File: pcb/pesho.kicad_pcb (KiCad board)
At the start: 2 copper layers, 132.5 x 65 mm, 60 parts, among them IC1 4N25, IC2 4N25, IC3 4N25, IC4 4N25, IC5 4N25, IC6 4N25, P1 Power, P2 Bulkey, P3 Raspberry Pi CONN, P4 Serial, U1 JE-112D, U2 JE-112D, U3 JE-112D

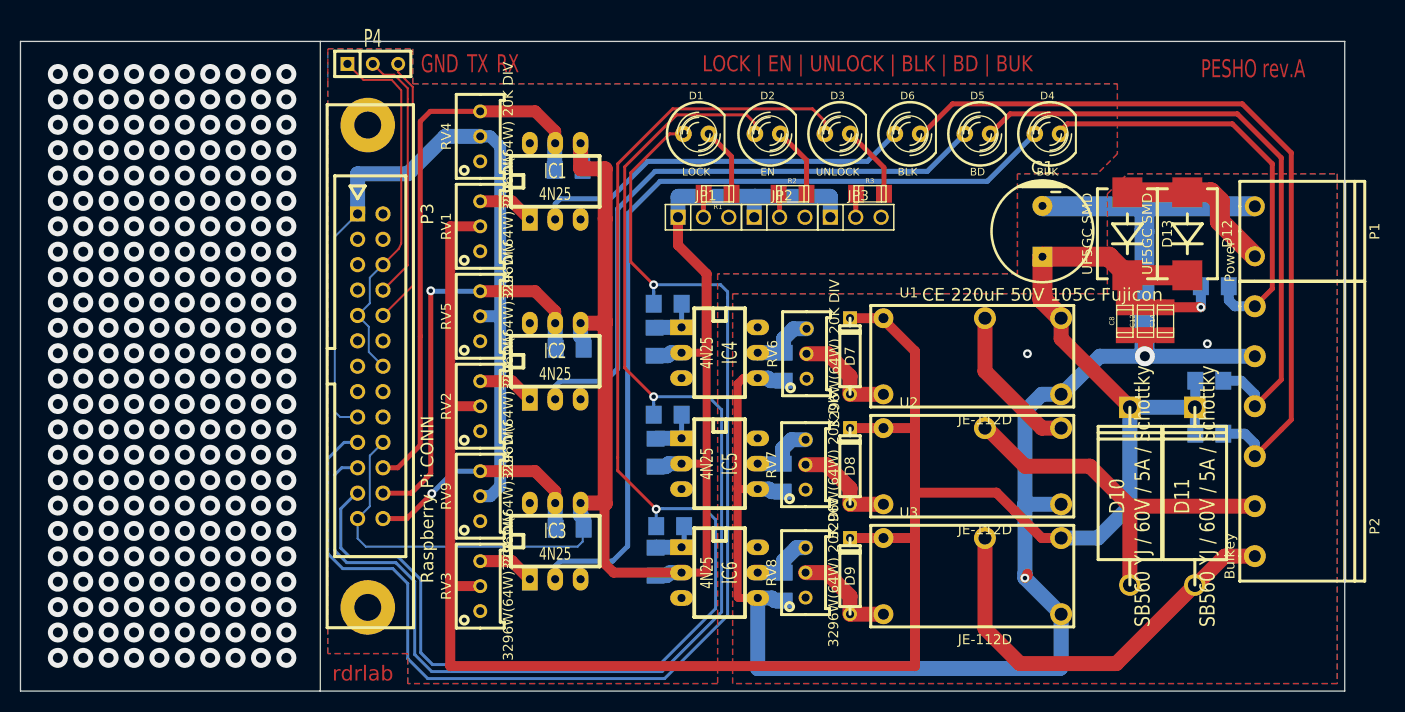
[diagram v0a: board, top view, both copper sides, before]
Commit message: Last version with fixed drills and send for production.
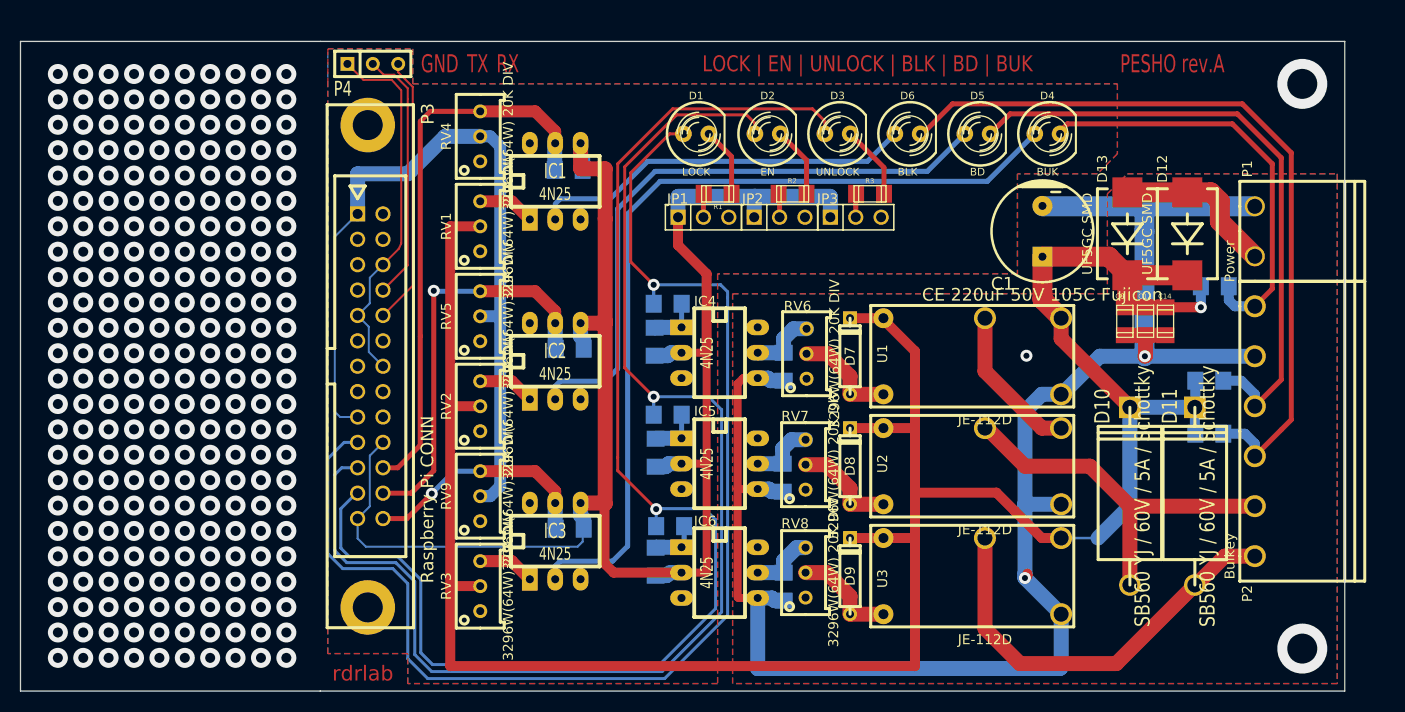
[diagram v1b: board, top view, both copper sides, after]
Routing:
- net GNDA: vias 2 -> 3
